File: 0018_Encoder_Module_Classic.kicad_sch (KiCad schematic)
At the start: 6 parts, among them U1 ENC_01, U2 ENC_02

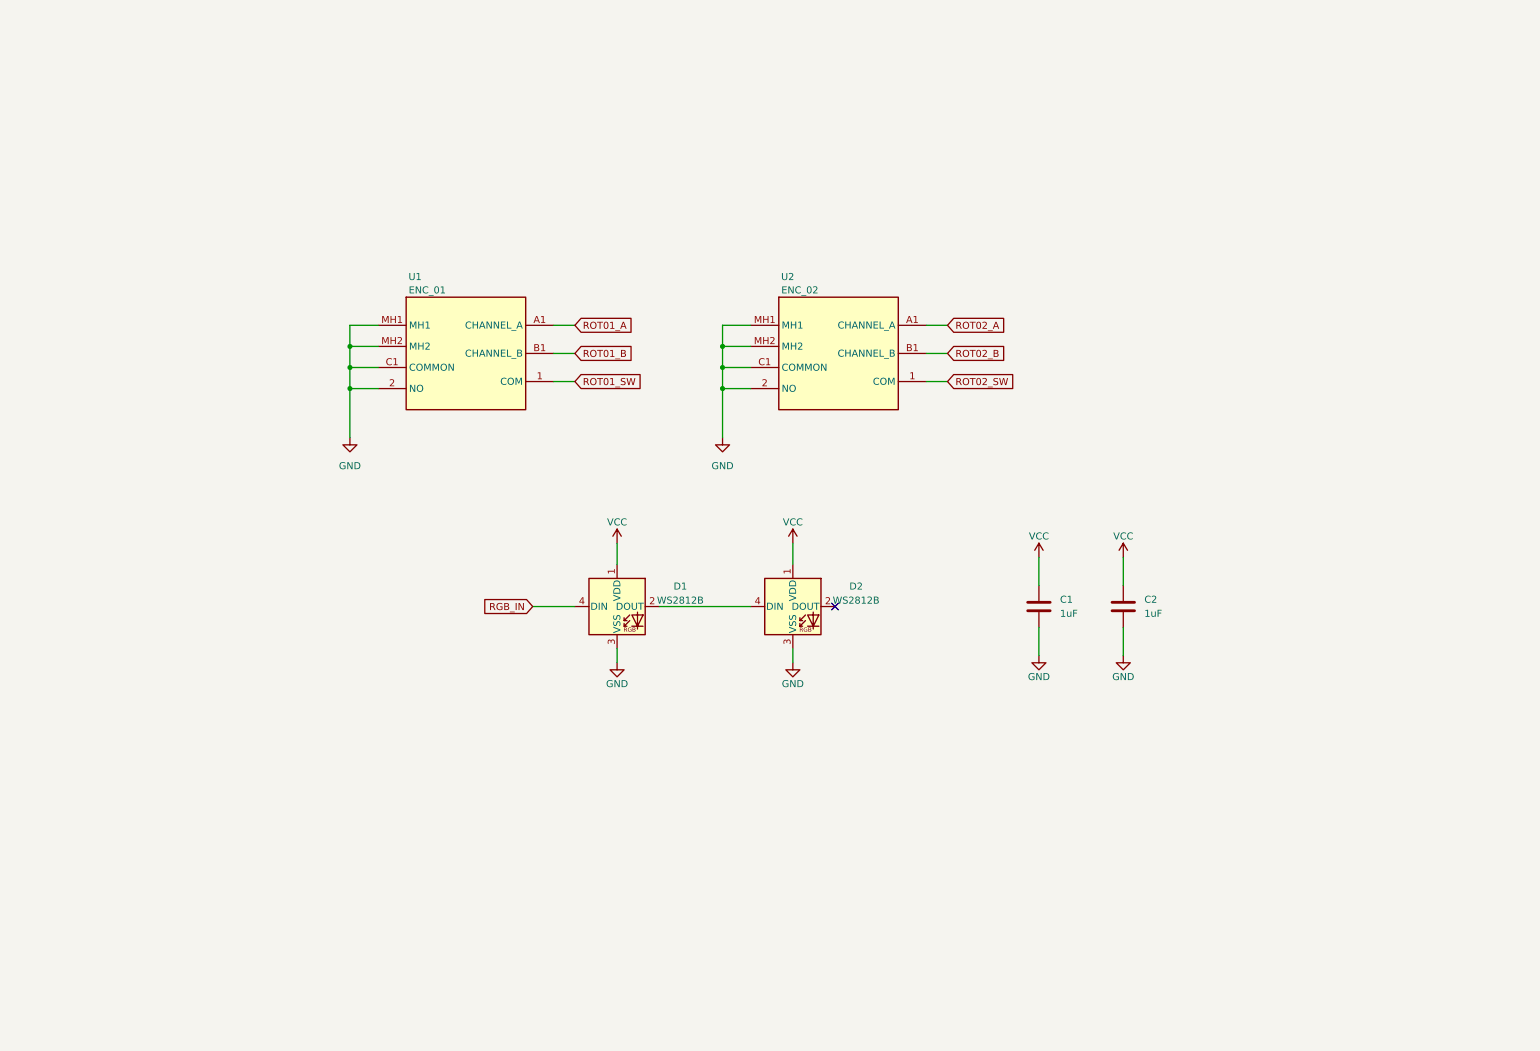
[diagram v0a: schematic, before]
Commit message: Add files via upload
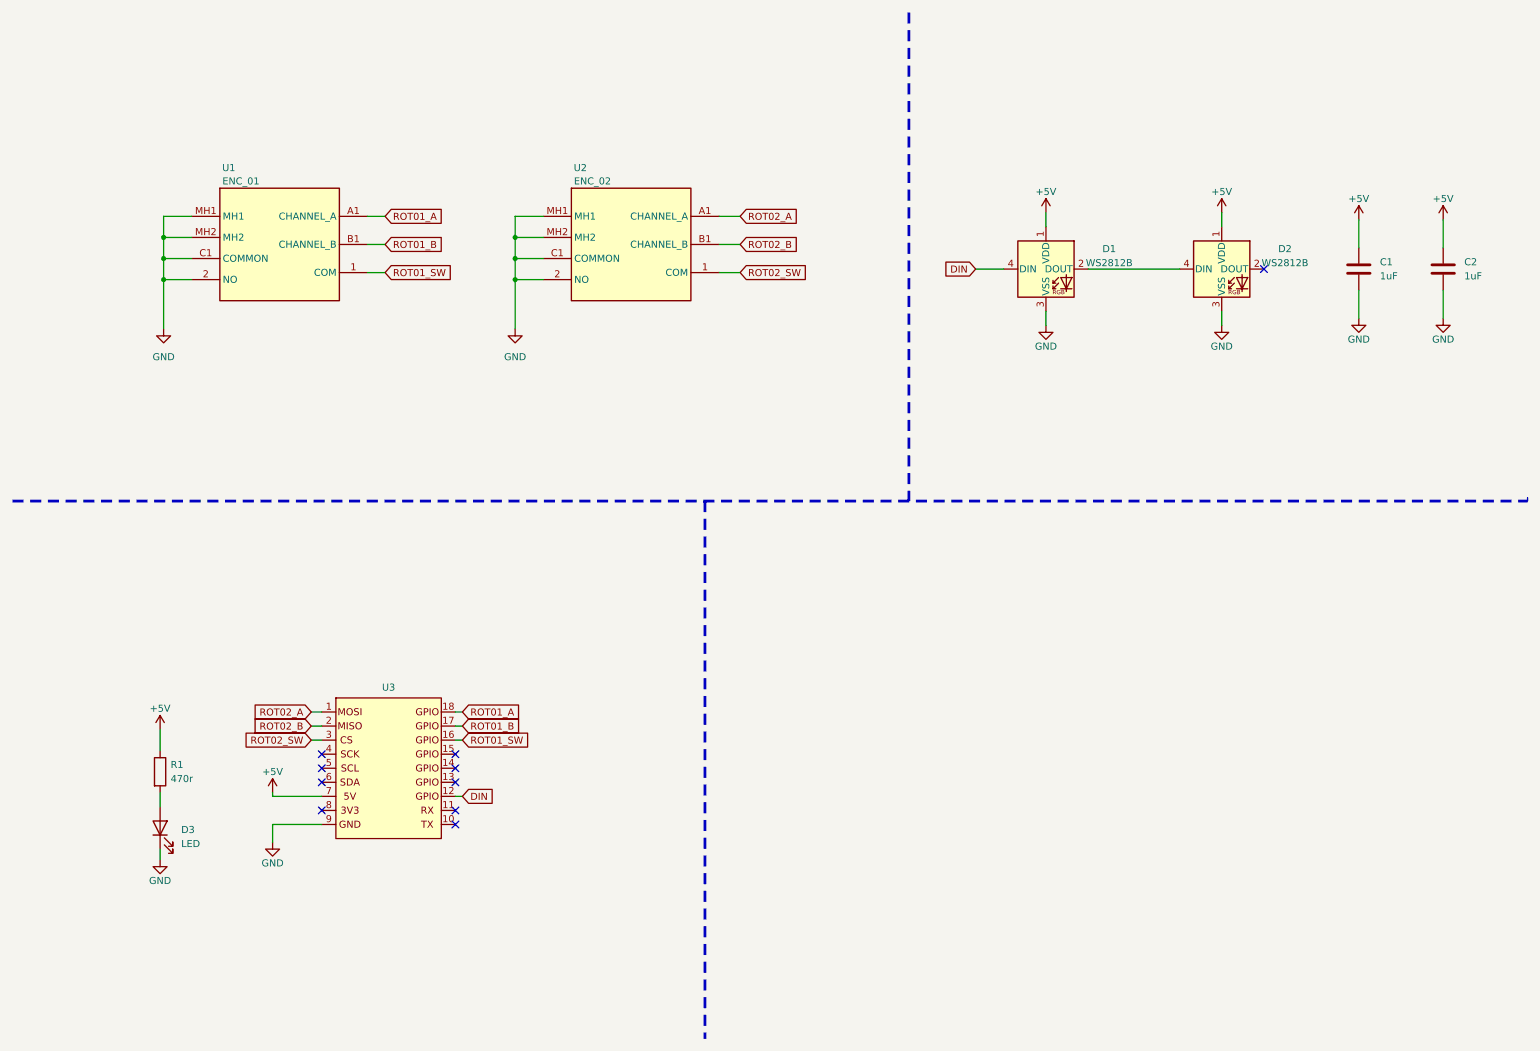
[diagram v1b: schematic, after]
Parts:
- added D3: LED, LED_SMD:LED_0603_1608Metric, symbol Device:LED
- added R1: 470r, Resistor_SMD:R_0603_1608Metric, symbol Device:R
- added U3: ~, Moduler_:pin_header_5-3, symbol moduler_pin:air
- C1, C2: footprint (none) -> Capacitor_SMD:C_0603_1608Metric
- U1, U2: footprint PEC11R4215FS0024 -> encoder:PEC11R4215FS0024
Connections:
- net GND: now also D3.1 (K), U3.9
- net ROT01_A: now also U3.18
- net ROT01_B: now also U3.17
- net ROT01_SW: now also U3.16
- net ROT02_A: now also U3.1
- net ROT02_B: now also U3.2
- net ROT02_SW: now also U3.3
- net RGB_IN renamed DIN
- net DIN: now also U3.12
- net VCC renamed +5V
- net +5V: now also R1.1, U3.7
- new net: D3.2 (A), R1.2
- no-connect marks 1 -> 10
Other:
- moved on the sheet: C1, C2, D1, D2, U1, U2
